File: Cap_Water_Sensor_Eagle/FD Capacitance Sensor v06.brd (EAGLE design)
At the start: 160 x 100 mm, 17 parts, among them U1 NTS4101PT1, U2 TLC555CD

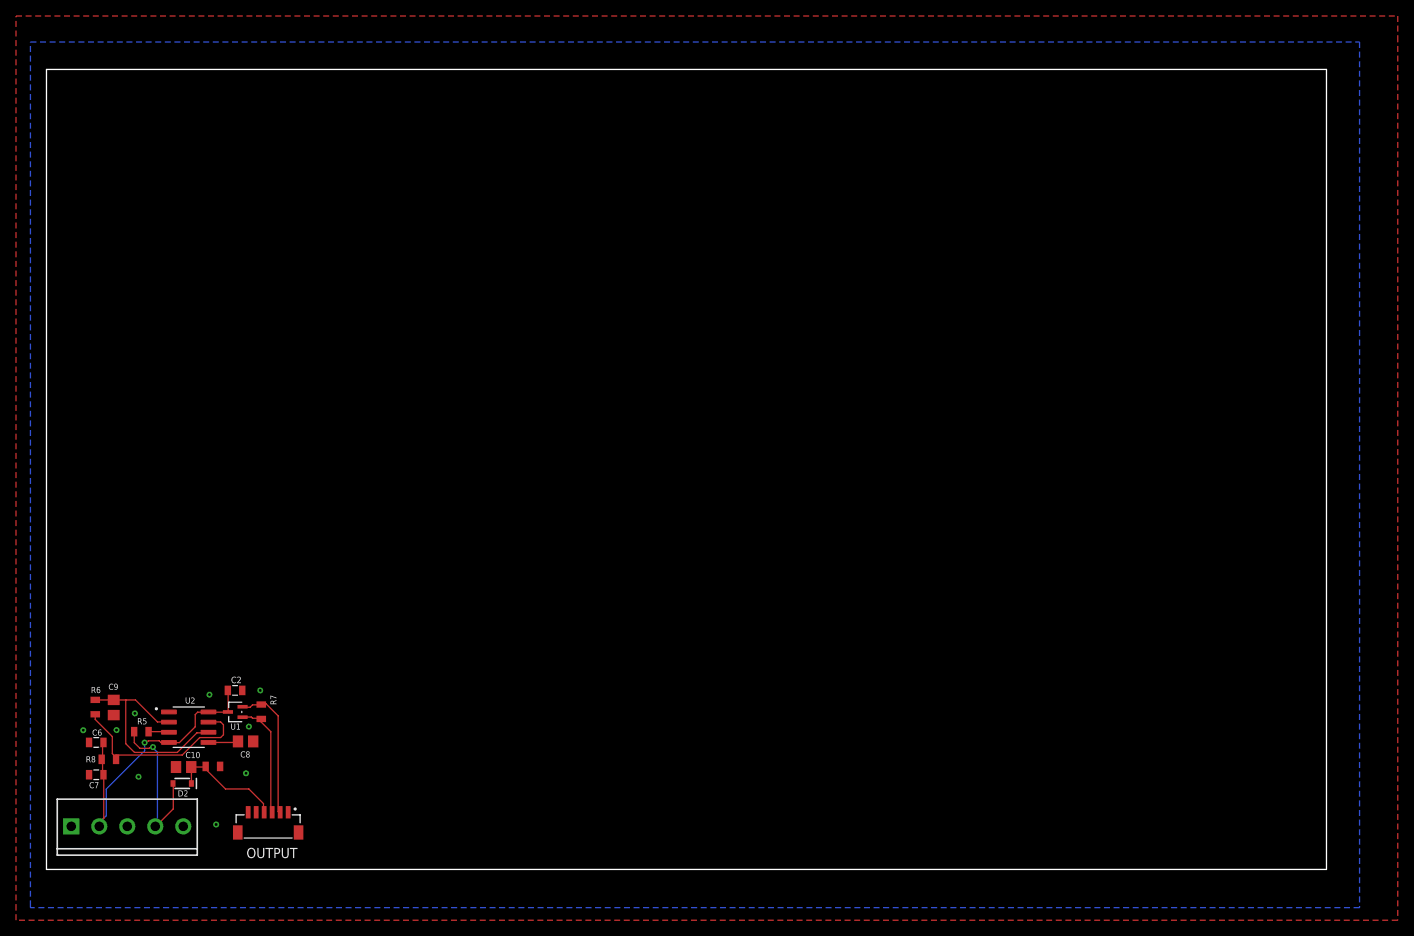
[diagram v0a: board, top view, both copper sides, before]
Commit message: Newest BRD
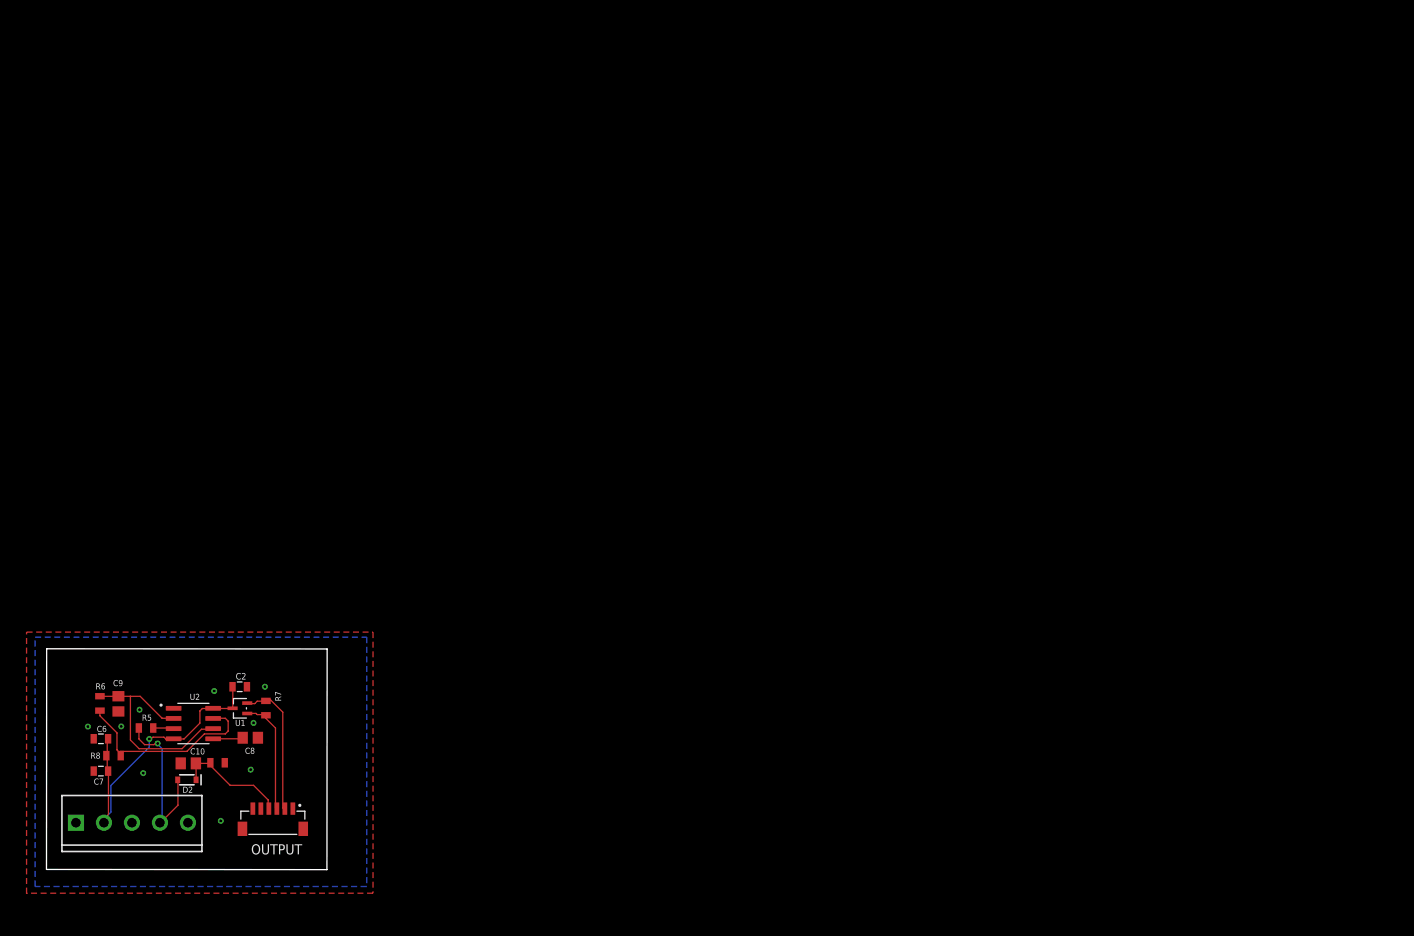
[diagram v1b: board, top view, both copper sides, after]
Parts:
- removed FRAME1: FRAME-LETTERNO_PACKAGE, SparkFun-Aesthetics:DUMMY
- moved D2 0.74 mm to (17.6, 11.2)
- moved U1 0.74 mm to (24.2, 20.1)
- moved C6 0.74 mm to (6.81, 16.3)
- moved C7 0.74 mm to (6.81, 12.3)
- moved R6 0.74 mm to (6.68, 20.8)
- moved R8 0.74 mm to (8.38, 14.2)
- moved C10 0.74 mm to (17.7, 13.3)
- moved C8 0.74 mm to (25.5, 16.5)
- moved C9 0.74 mm to (8.99, 20.7)
- moved OUTPUT 0.74 mm to (28.3, 5.08)
- moved R5 0.74 mm to (12.4, 17.7)
- moved R7 0.74 mm to (27.4, 20.2)
- moved R9 0.74 mm to (21.4, 13.3)
- moved U2 0.74 mm to (18.4, 18.2)
- moved J1 0.74 mm to (3.68, 5.84)
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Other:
- board size 160 x 100 mm -> 35.1 x 27.6 mm
